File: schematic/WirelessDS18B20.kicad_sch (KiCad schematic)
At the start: 8 parts, among them P1 1-Wire Bus, Q1 2N7002, U1 WeMos_mini, U2 AMS1117-3.3

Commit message: Update schematic
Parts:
- C1: LCSC C119052 -> C7171
- C2: LCSC C129289 -> C16133
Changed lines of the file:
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@@
 			)
 		)
-		(property "LCSC" "C119052"
+		(property "LCSC" "C7171"
 			(at 22.86 66.04 0)
 			(effects
@@
 			)
 		)
-		(property "LCSC" "C129289"
+		(property "LCSC" "C16133"
 			(at 44.45 66.04 0)
 			(effects

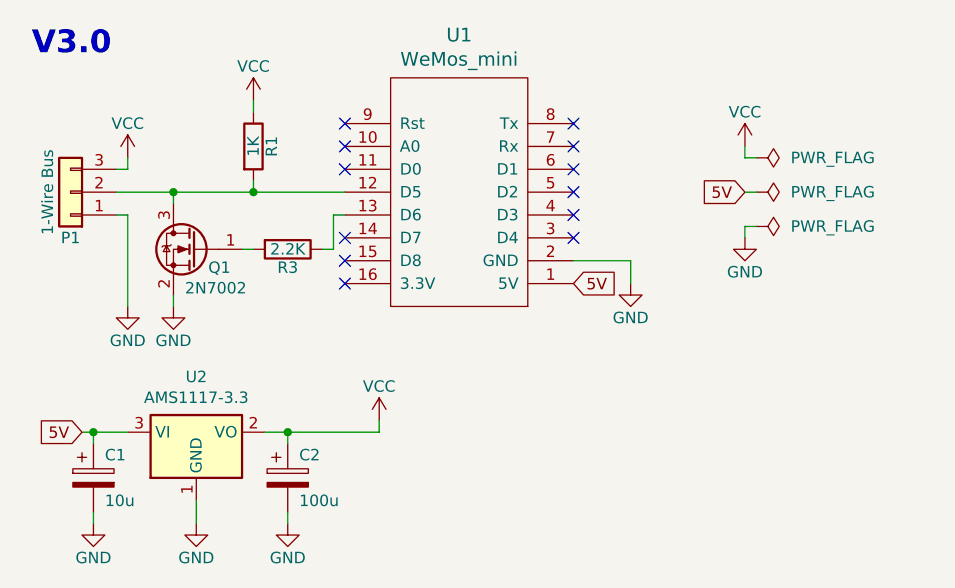
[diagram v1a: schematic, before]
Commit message: Update schematic
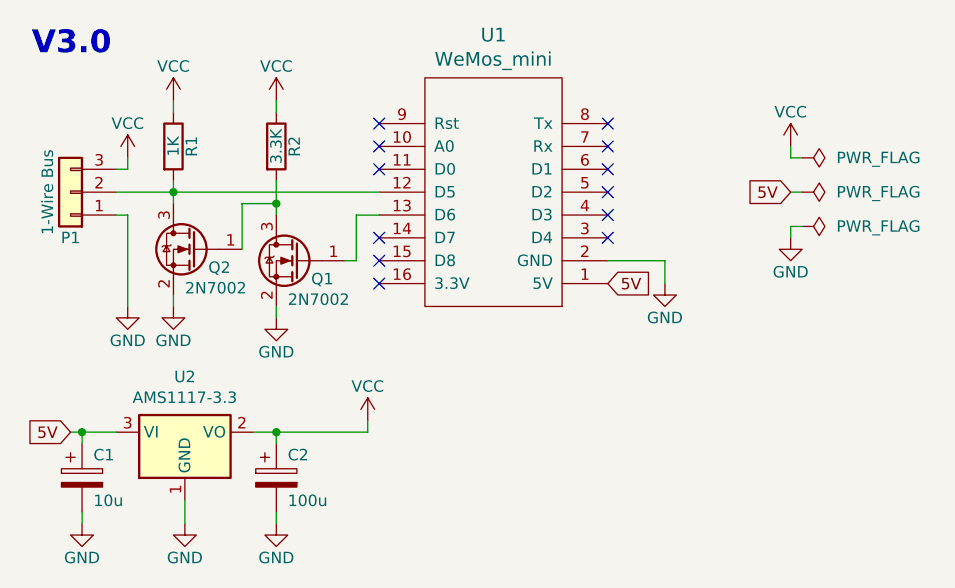
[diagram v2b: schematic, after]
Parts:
- added Q2: 2N7002, Package_TO_SOT_SMD:SOT-23_Handsoldering, symbol Transistor_FET:2N7002
- R2: renamed from R3; value 2.2K -> 3.3K; LCSC C17520 -> C26010
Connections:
- net GND: now also Q2.2 (S)
- net VCC: now also R2.1
- net at P1.2 (Pin_2), R1.2, U1.12 (D5): now also Q2.3 (D); no longer Q1.3 (D)
- net at U1.13 (D6): now also Q1.1 (G); no longer R2.1
- net at R2.2: now also Q1.3 (D), Q2.1 (G); no longer Q1.1 (G)
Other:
- moved on the sheet: C1, C2, Q1, R1, R2, U1, U2
